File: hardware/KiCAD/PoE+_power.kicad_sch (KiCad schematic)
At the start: 69 parts, among them Q2 FDMC2523P, Q3 FDS86242, Q4 CSD19534Q, Q5 FCX493, Q6 FCX493, Q7 CSD19534Q, T1 PA4065NL, U5 TPS23754, U6 HMHA2801A, U7 PC357N

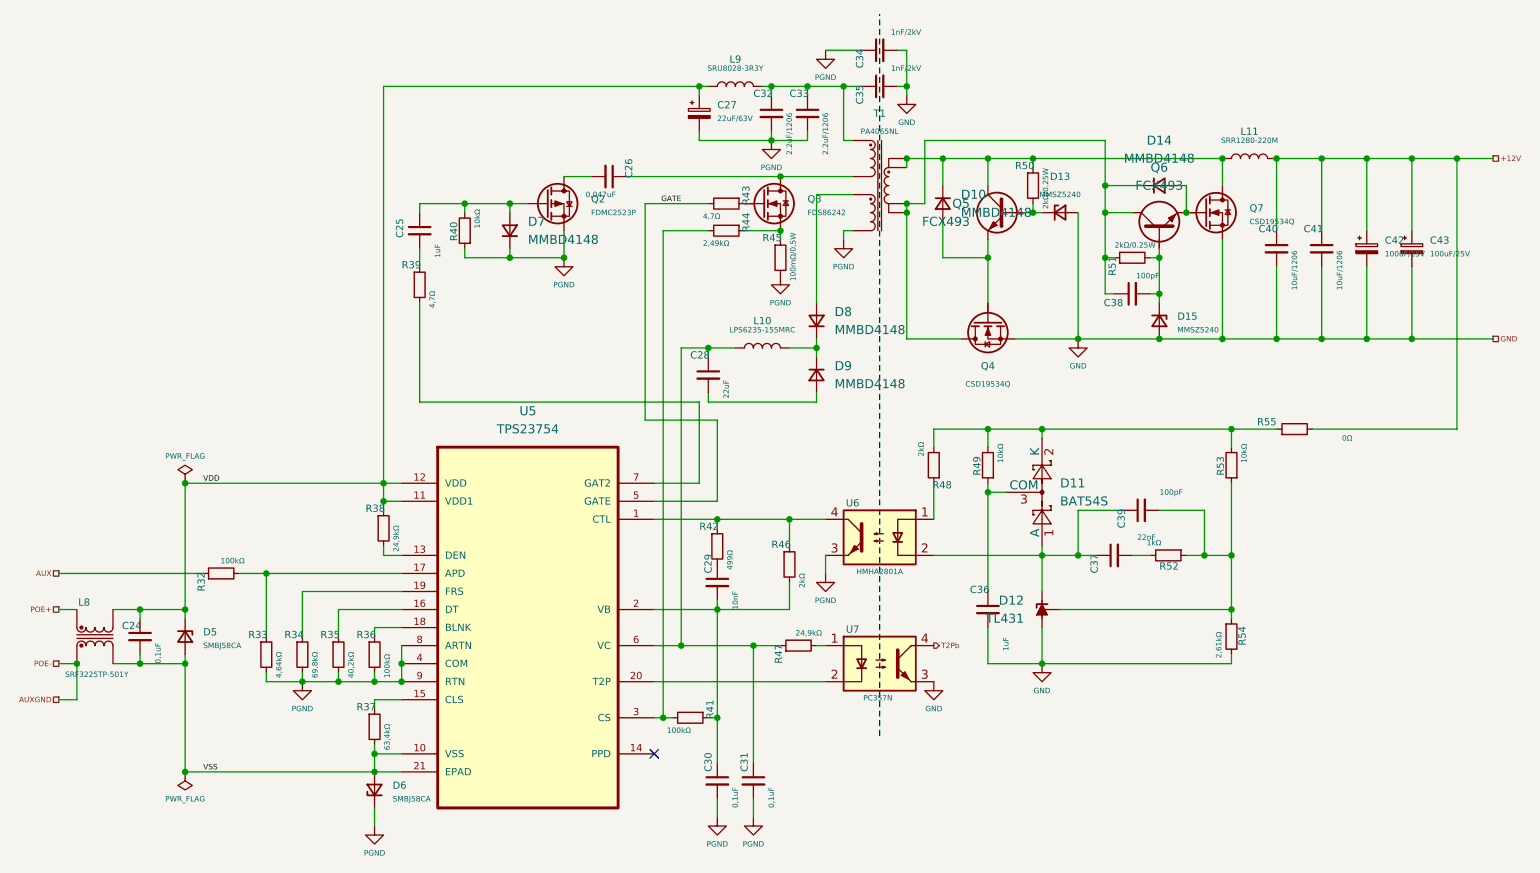
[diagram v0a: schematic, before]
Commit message: update
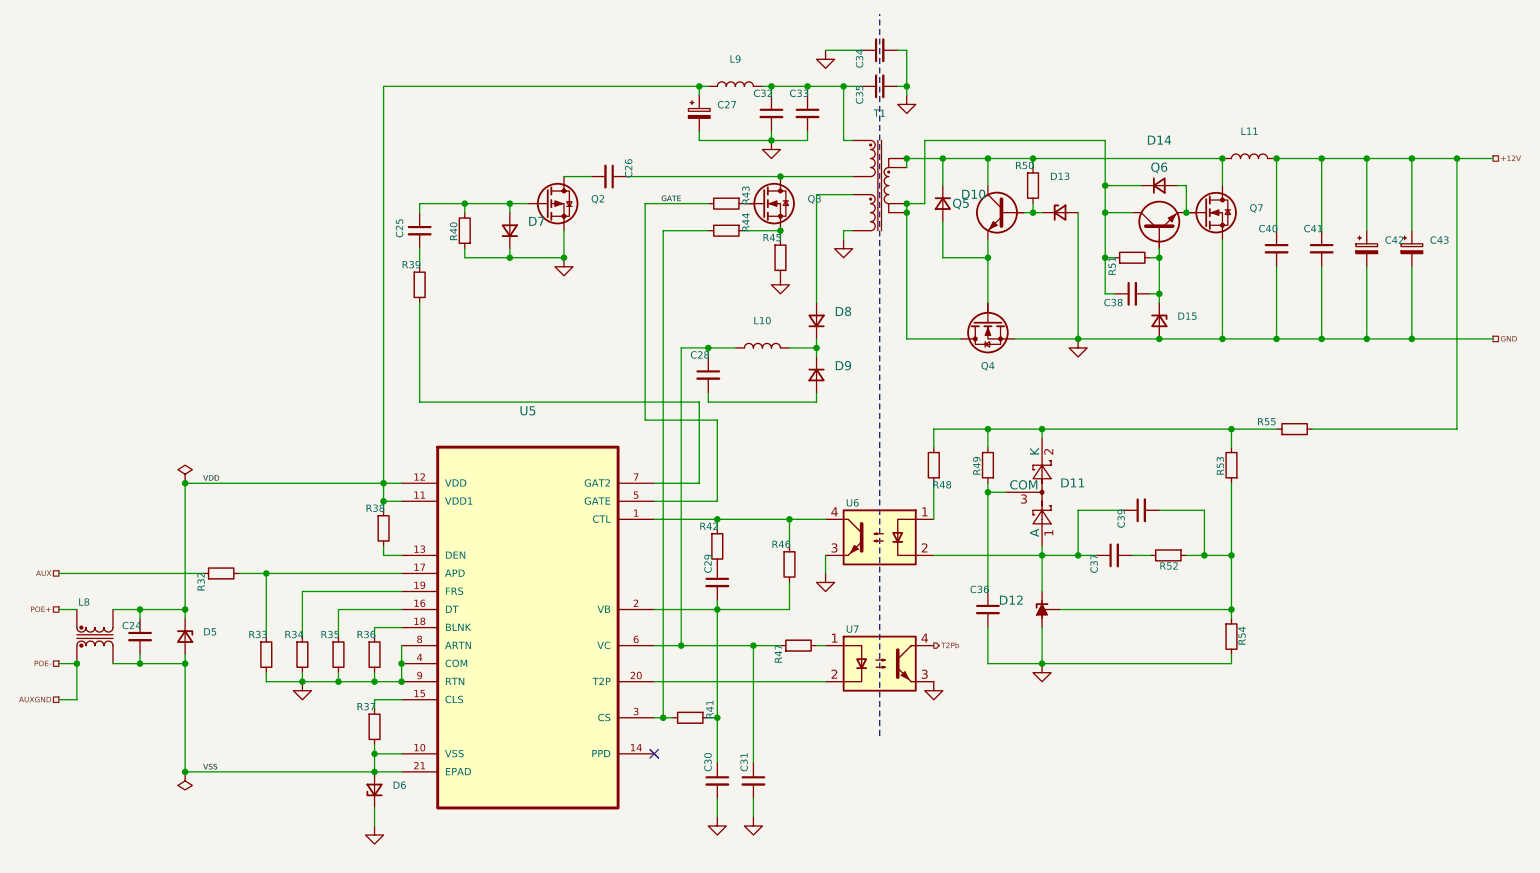
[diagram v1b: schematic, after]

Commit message: update
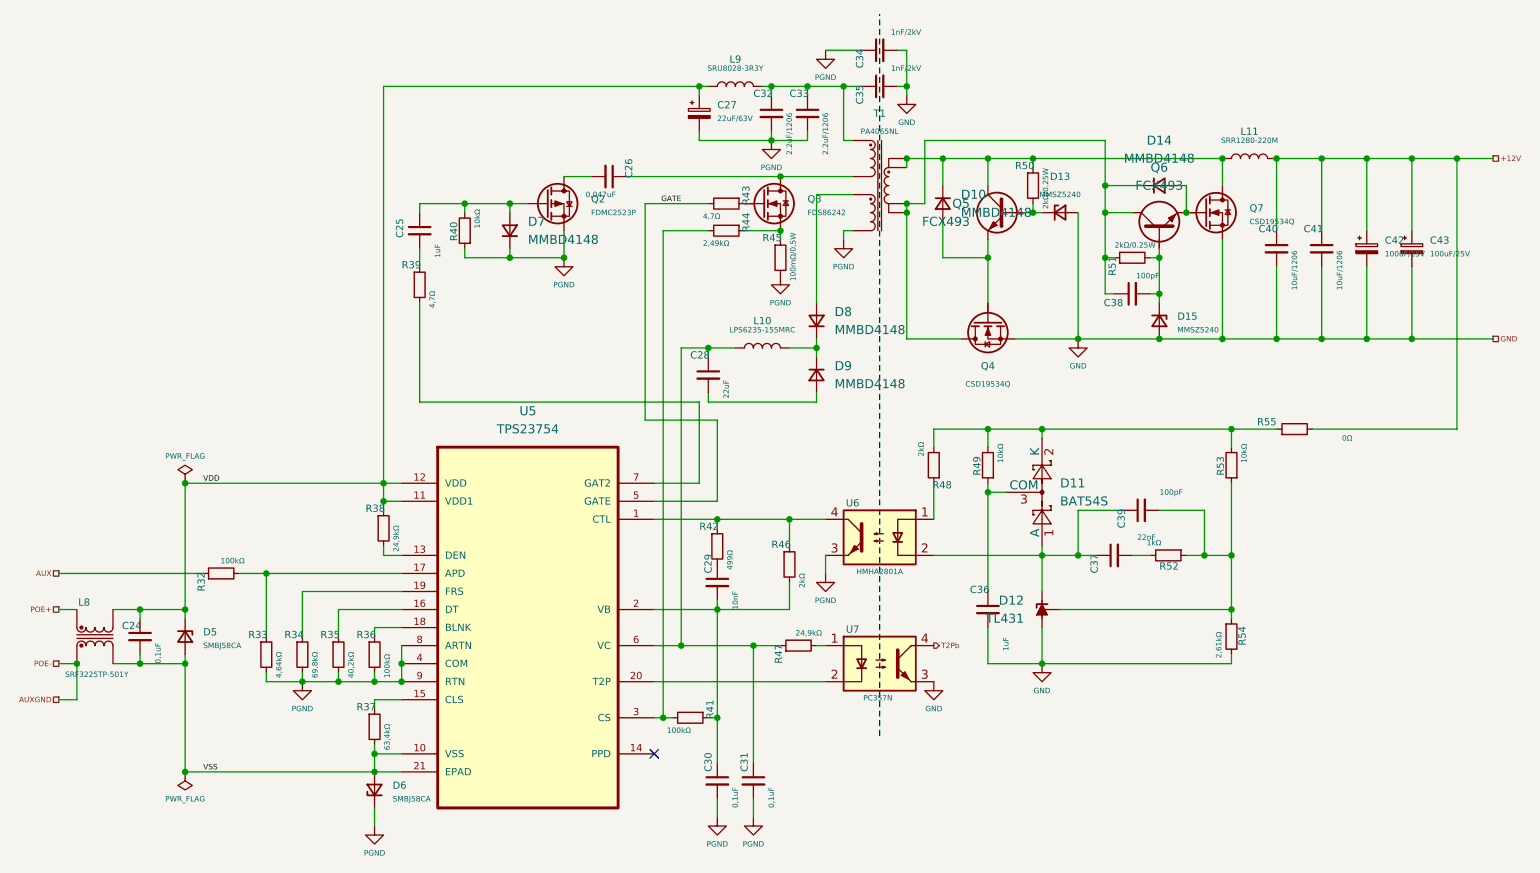
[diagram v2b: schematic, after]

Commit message: update
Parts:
- U7: footprint Package_SO:SOIC-4_4.55x3.7mm_P2.54mm -> Package_SO:OnSemi_751EP_SOIC-4_3.9x4.725mm_P2.54mm
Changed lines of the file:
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@@
 			)
 		)
-		(property "Footprint" "Package_SO:SOIC-4_4.55x3.7mm_P2.54mm"
+		(property "Footprint" "Package_SO:OnSemi_751EP_SOIC-4_3.9x4.725mm_P2.54mm"
 			(at 157.48 129.54 0)
 			(effects
